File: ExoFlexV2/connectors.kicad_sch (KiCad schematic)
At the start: 12 parts, among them J10 Conn_01x03_Male, J11 Conn_01x05_Male, J12 Conn_01x03_Male, J13 Conn_01x05_Male, J14 Conn_01x03_Male, J15 Conn_01x04_Male, J16 Conn_01x09_Male, J17 Conn_01x08_Male, J18 Conn_01x04_Male, J19 Conn_01x09_Male, J8 Conn_01x03_Male, J9 Conn_01x05_Male

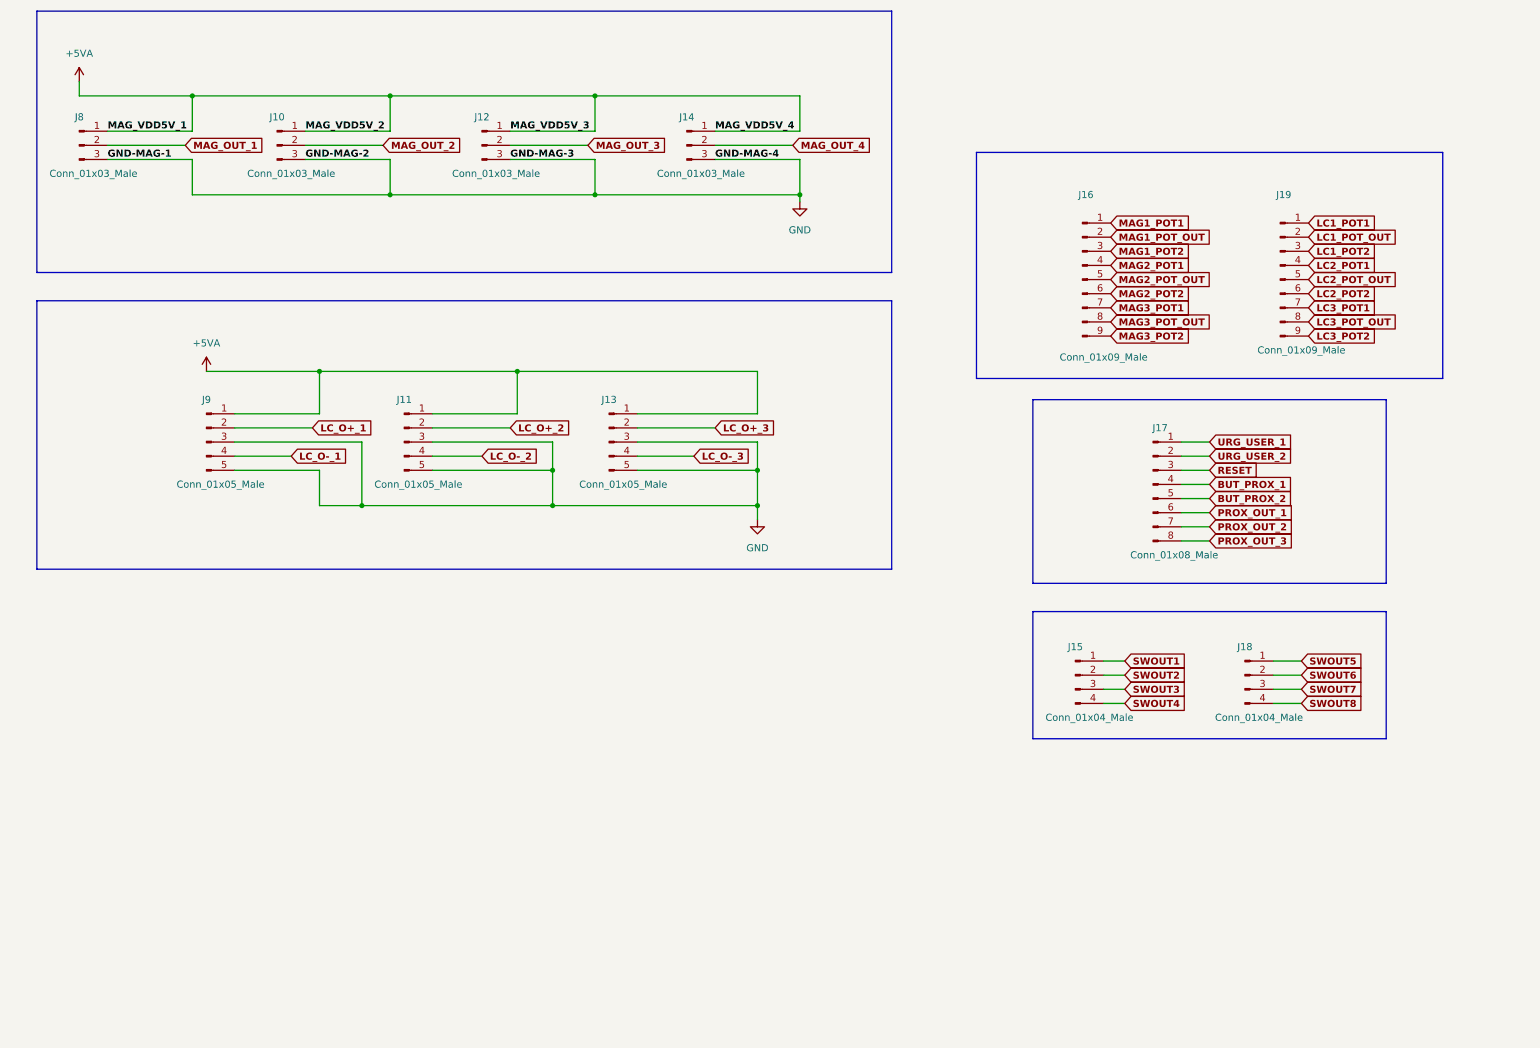
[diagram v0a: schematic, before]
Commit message: quque truc
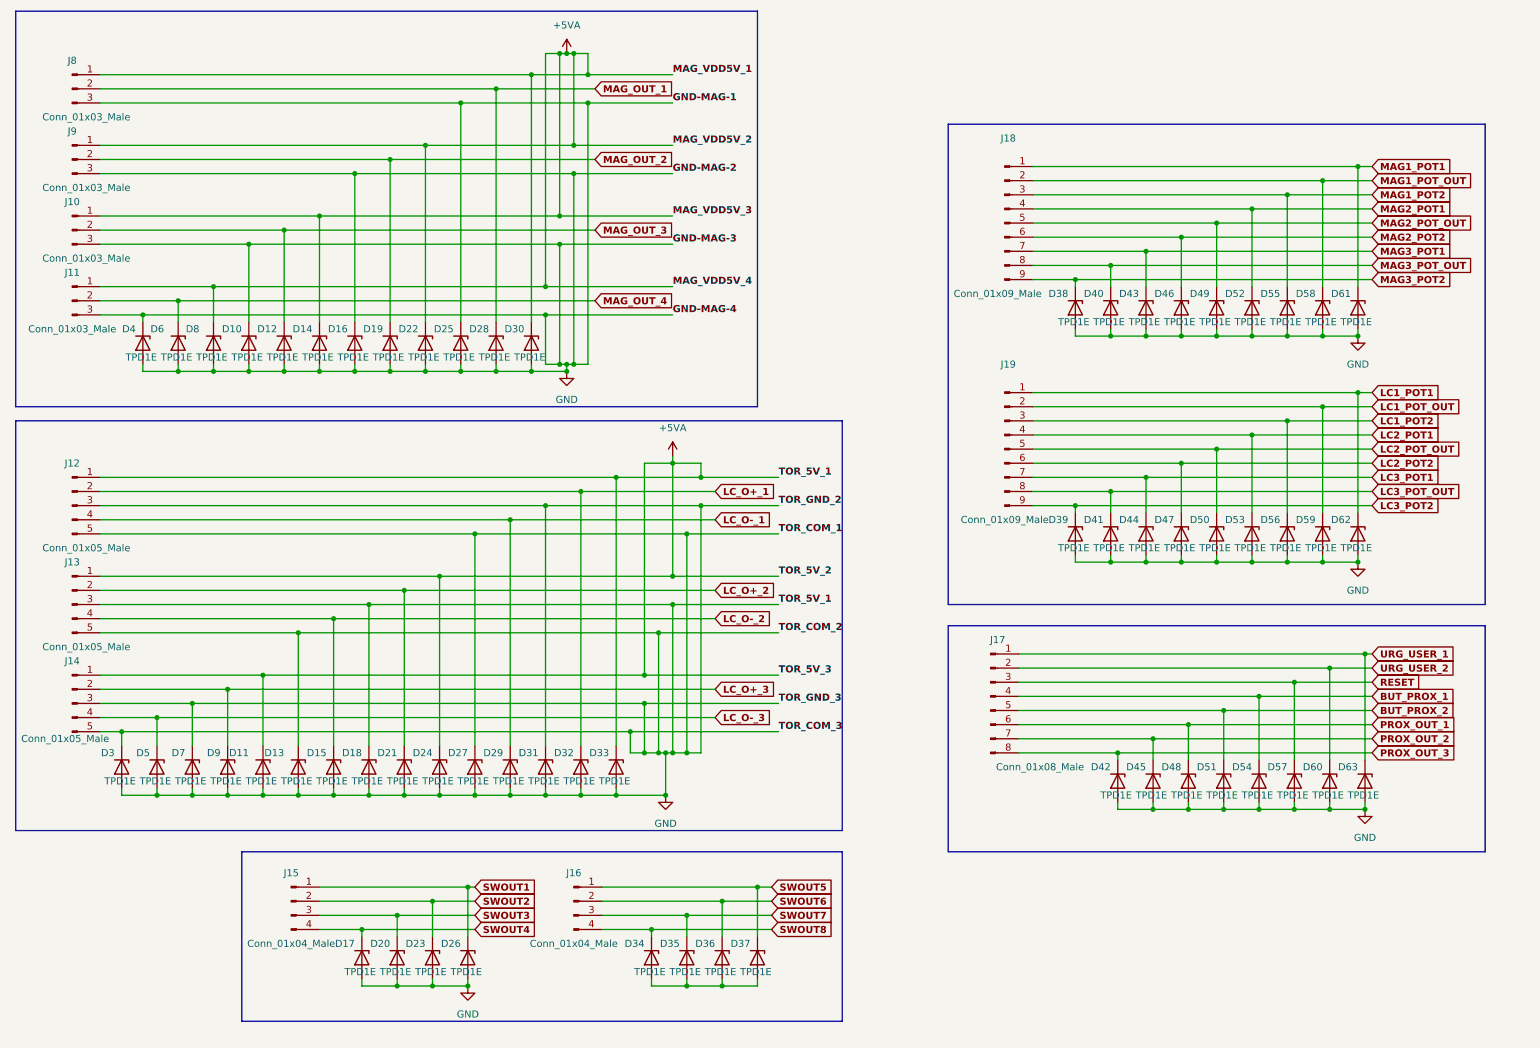
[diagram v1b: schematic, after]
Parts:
- added D10, D11, D12, D13, D14, D15, D16, D17, D18, D19, D20, D21, D22, D23, D24, D25, D26, D27, D28, D29, D3, D30, D31, D32, D33, D34, D35, D36, D37, D38, D39, D4, D40, D41, D42, D43, D44, D45, D46, D47, D48, D49, D5, D50, D51, D52, D53, D54, D55, D56, D57, D58, D59, D6, D60, D61, D62, D63, D7, D8, D9: TPD1E, FootPrint:DPY2_TEX, symbol Device:D_Zener
- J12: renamed from J9; footprint (none) -> Connector_PinHeader_2.54mm:PinHeader_1x05_P2.54mm_Vertical
- J13: renamed from J11; footprint (none) -> Connector_PinHeader_2.54mm:PinHeader_1x05_P2.54mm_Vertical
- J14: renamed from J13; footprint (none) -> Connector_PinHeader_2.54mm:PinHeader_1x05_P2.54mm_Vertical
- renumbered J12 to J10, J14 to J11, J18 to J16, J16 to J18, J10 to J9
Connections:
- net GND is gone; now on net +5VA: J10.3 (Pin_3), J11.3 (Pin_3), J12.3 (Pin_3), J12.5 (Pin_5), J13.3 (Pin_3), J13.5 (Pin_5), J14.3 (Pin_3), J14.5 (Pin_5), J8.3 (Pin_3), J9.3 (Pin_3)
- net +5VA: now also D10.1 (K), D10.2 (A), D11.1 (K), D11.2 (A), D12.2 (A), D13.1 (K), D13.2 (A), D14.1 (K), D14.2 (A), D15.2 (A), D16.1 (K), D16.2 (A), D17.2 (A), D18.1 (K), D18.2 (A), D19.2 (A), D20.2 (A), D21.2 (A), D22.1 (K), D22.2 (A), D23.2 (A), D24.1 (K), D24.2 (A), D25.1 (K), D25.2 (A), D26.2 (A), D27.1 (K), D27.2 (A), D28.2 (A), D29.2 (A), D3.1 (K), D3.2 (A), D30.1 (K), D30.2 (A), D31.1 (K), D31.2 (A), D32.2 (A), D33.1 (K), D33.2 (A), D38.2 (A), D39.2 (A), D4.1 (K), D4.2 (A), D40.2 (A), D41.2 (A), D42.2 (A), D43.2 (A), D44.2 (A), D45.2 (A), D46.2 (A), D47.2 (A), D48.2 (A), D49.2 (A), D5.2 (A), D50.2 (A), D51.2 (A), D52.2 (A), D53.2 (A), D54.2 (A), D55.2 (A), D56.2 (A), D57.2 (A), D58.2 (A), D59.2 (A), D6.2 (A), D60.2 (A), D61.2 (A), D62.2 (A), D63.2 (A), D7.1 (K), D7.2 (A), D8.1 (K), D8.2 (A), D9.2 (A)
- net BUT_PROX_1: now also D54.1 (K)
- net BUT_PROX_2: now also D51.1 (K)
- net LC1_POT1: now also D62.1 (K)
- net LC1_POT2: now also D56.1 (K)
- net LC1_POT_OUT: now also D59.1 (K)
- net LC2_POT1: now also D53.1 (K)
- net LC2_POT2: now also D47.1 (K)
- net LC2_POT_OUT: now also D50.1 (K)
- net LC3_POT1: now also D44.1 (K)
- net LC3_POT2: now also D39.1 (K)
- net LC3_POT_OUT: now also D41.1 (K)
- net LC_O+_1: now also D32.1 (K)
- net LC_O+_2: now also D21.1 (K)
- net LC_O+_3: now also D9.1 (K)
- net LC_O-_1: now also D29.1 (K)
- net LC_O-_2: now also D15.1 (K)
- net LC_O-_3: now also D5.1 (K)
- net MAG1_POT1: now also D61.1 (K)
- net MAG1_POT2: now also D55.1 (K)
- net MAG1_POT_OUT: now also D58.1 (K)
- net MAG2_POT1: now also D52.1 (K)
- net MAG2_POT2: now also D46.1 (K)
- net MAG2_POT_OUT: now also D49.1 (K)
- net MAG3_POT1: now also D43.1 (K)
- net MAG3_POT2: now also D38.1 (K)
- net MAG3_POT_OUT: now also D40.1 (K)
- net MAG_OUT_1: now also D28.1 (K)
- net MAG_OUT_2: now also D19.1 (K)
- net MAG_OUT_3: now also D12.1 (K)
- net MAG_OUT_4: now also D6.1 (K)
- net PROX_OUT_1: now also D48.1 (K)
- net PROX_OUT_2: now also D45.1 (K)
- net PROX_OUT_3: now also D42.1 (K)
- net RESET: now also D57.1 (K)
- net SWOUT1: now also D26.1 (K)
- net SWOUT2: now also D23.1 (K)
- net SWOUT3: now also D20.1 (K)
- net SWOUT4: now also D17.1 (K)
- net SWOUT5: now also D37.1 (K)
- net SWOUT6: now also D36.1 (K)
- net SWOUT7: now also D35.1 (K)
- net SWOUT8: now also D34.1 (K)
- net URG_USER_1: now also D63.1 (K)
- net URG_USER_2: now also D60.1 (K)
- new net: D34.2 (A), D35.2 (A), D36.2 (A), D37.2 (A)
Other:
- moved on the sheet: J10, J11, J12, J13, J14, J15, J16, J17, J18, J19, J8, J9

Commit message: Placement
Début du placement et modification d'après dernier review
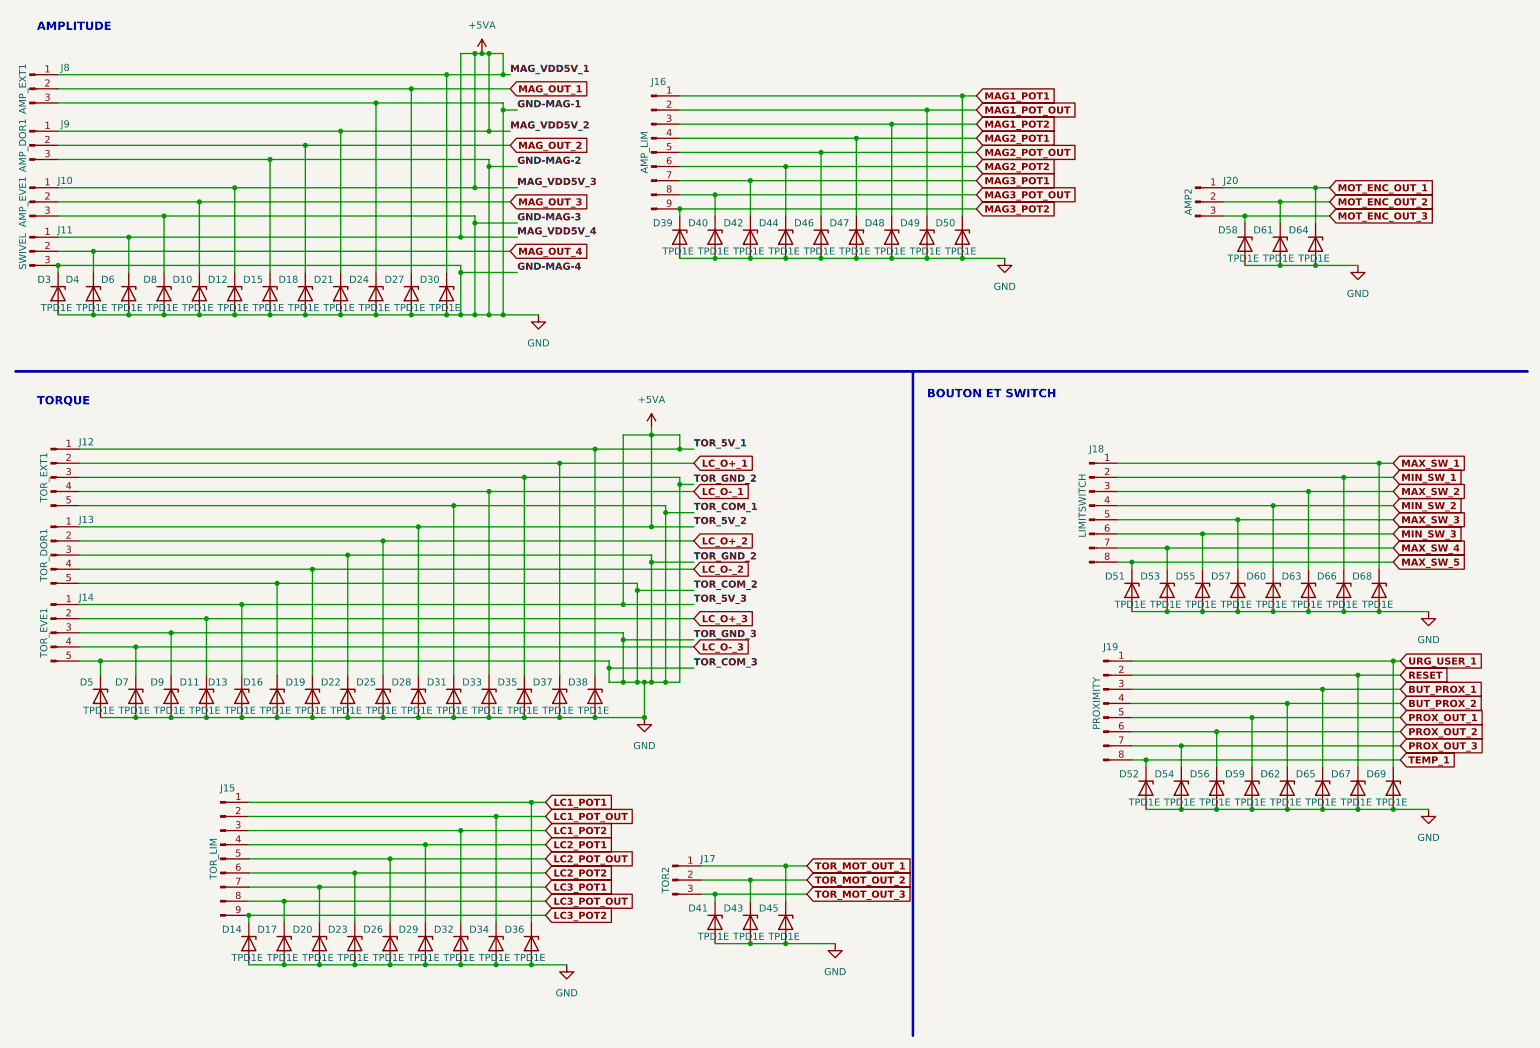
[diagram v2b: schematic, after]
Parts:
- removed D17, D20, D23, D26, D34, D35, D36, D37: TPD1E, FootPrint:DPY2_TEX, symbol Device:D_Zener
- removed J15, J16: Conn_01x04_Male, Connector_PinHeader_2.54mm:PinHeader_1x04_P2.54mm_Vertical, symbol Connector:Conn_01x04_Male
- added D41, D43, D45, D51, D53, D55, D57, D58, D60, D61, D63, D64, D66, D68: TPD1E, FootPrint:DPY2_TEX, symbol Device:D_Zener
- added J17: TOR2, Connector_PinHeader_2.54mm:PinHeader_1x03_P2.54mm_Vertical, symbol Connector:Conn_01x03_Male
- added J18: LIMITSWITCH, Connector_PinHeader_2.54mm:PinHeader_1x08_P2.54mm_Vertical, symbol Connector:Conn_01x08_Male
- added J20: AMP2, Connector_PinHeader_2.54mm:PinHeader_1x03_P2.54mm_Vertical, symbol Connector:Conn_01x03_Male
- J10: value Conn_01x03_Male -> AMP_EVE1
- J11: value Conn_01x03_Male -> SWIVEL
- J12: value Conn_01x05_Male -> TOR_EXT1
- J13: value Conn_01x05_Male -> TOR_DOR1
- J14: value Conn_01x05_Male -> TOR_EVE1
- J15: renamed from J19; value Conn_01x09_Male -> TOR_LIM
- J16: renamed from J18; value Conn_01x09_Male -> AMP_LIM
- J19: renamed from J17; value Conn_01x08_Male -> PROXIMITY
- J8: value Conn_01x03_Male -> AMP_EXT1
- J9: value Conn_01x03_Male -> AMP_DOR1
- renumbered D12 to D10, D9 to D11, D14 to D12, D11 to D13, D39 to D14, D16 to D15, D13 to D16, D41 to D17, D19 to D18, D15 to D19, D44 to D20, D22 to D21, D18 to D22, D47 to D23, D25 to D24, D21 to D25, D50 to D26, D28 to D27, D24 to D28, D53 to D29, D4 to D3, D27 to D31, D56 to D32, D29 to D33, D59 to D34, D31 to D35, D62 to D36, D32 to D37, D33 to D38, D38 to D39, D6 to D4, D43 to D42, D46 to D44, D49 to D46, D52 to D47, D55 to D48, D58 to D49, D3 to D5, D61 to D50, D42 to D52, D45 to D54, D48 to D56, D51 to D59, D8 to D6, D54 to D62, D57 to D65, D60 to D67, D63 to D69, D5 to D7, D10 to D8, D7 to D9
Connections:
- net URG_USER_2 is gone; now on net RESET: D67.1 (K), J19.2 (Pin_2)
- net +5VA: no longer D10.2 (A), D11.2 (A), D12.2 (A), D13.2 (A), D14.2 (A), D15.1 (K), D15.2 (A), D16.1 (K), D16.2 (A), D17.2 (A), D18.2 (A), D19.2 (A), D20.2 (A), D21.2 (A), D22.1 (K), D22.2 (A), D23.2 (A), D24.1 (K), D24.2 (A), D25.2 (A), D26.2 (A), D27.2 (A), D28.2 (A), D29.2 (A), D3.1 (K), D3.2 (A), D30.2 (A), D31.1 (K), D31.2 (A), D32.2 (A), D33.2 (A), D34.2 (A), D35.1 (K), D35.2 (A), D36.2 (A), D37.2 (A), D38.2 (A), D39.2 (A), D4.2 (A), D40.2 (A), D42.2 (A), D44.2 (A), D46.2 (A), D47.2 (A), D48.2 (A), D49.2 (A), D5.1 (K), D5.2 (A), D50.2 (A), D52.2 (A), D54.2 (A), D56.2 (A), D59.2 (A), D6.2 (A), D62.2 (A), D65.2 (A), D67.2 (A), D69.2 (A), D7.2 (A), D8.1 (K), D8.2 (A), D9.1 (K), D9.2 (A), J10.3 (Pin_3), J11.3 (Pin_3), J12.3 (Pin_3), J12.5 (Pin_5), J13.3 (Pin_3), J13.5 (Pin_5), J14.3 (Pin_3), J14.5 (Pin_5), J8.3 (Pin_3), J9.3 (Pin_3)
- net BUT_PROX_1: now also D65.1 (K), J19.3 (Pin_3); no longer D62.1 (K), J19.4 (Pin_4)
- net BUT_PROX_2: now also D62.1 (K), J19.4 (Pin_4); no longer D59.1 (K), J19.5 (Pin_5)
- net PROX_OUT_1: now also D59.1 (K), J19.5 (Pin_5); no longer D56.1 (K), J19.6 (Pin_6)
- net PROX_OUT_2: now also D56.1 (K), J19.6 (Pin_6); no longer D54.1 (K), J19.7 (Pin_7)
- net PROX_OUT_3: now also D54.1 (K), J19.7 (Pin_7); no longer D52.1 (K), J19.8 (Pin_8)
- net RESET: no longer D65.1 (K), J19.3 (Pin_3)
- new net GND: D10.2 (A), D11.2 (A), D12.2 (A), D13.2 (A), D14.2 (A), D15.1 (K), D15.2 (A), D16.1 (K), D16.2 (A), D17.2 (A), D18.2 (A), D19.2 (A), D20.2 (A), D21.2 (A), D22.1 (K), D22.2 (A), D23.2 (A), D24.1 (K), D24.2 (A), D25.2 (A), D26.2 (A), D27.2 (A), D28.2 (A), D29.2 (A), D3.1 (K), D3.2 (A), D30.2 (A), D31.1 (K), D31.2 (A), D32.2 (A), D33.2 (A), D34.2 (A), D35.1 (K), D35.2 (A), D36.2 (A), D37.2 (A), D38.2 (A), D39.2 (A), D4.2 (A), D40.2 (A), D41.2 (A), D42.2 (A), D43.2 (A), D44.2 (A), D45.2 (A), D46.2 (A), D47.2 (A), D48.2 (A), D49.2 (A), D5.1 (K), D5.2 (A), D50.2 (A), D51.2 (A), D52.2 (A), D53.2 (A), D54.2 (A), D55.2 (A), D56.2 (A), D57.2 (A), D58.2 (A), D59.2 (A), D6.2 (A), D60.2 (A), D61.2 (A), D62.2 (A), D63.2 (A), D64.2 (A), D65.2 (A), D66.2 (A), D67.2 (A), D68.2 (A), D69.2 (A), D7.2 (A), D8.1 (K), D8.2 (A), D9.1 (K), D9.2 (A), J10.3 (Pin_3), J11.3 (Pin_3), J12.3 (Pin_3), J12.5 (Pin_5), J13.3 (Pin_3), J13.5 (Pin_5), J14.3 (Pin_3), J14.5 (Pin_5), J8.3 (Pin_3), J9.3 (Pin_3)
- new net MAX_SW_1: D68.1 (K), J18.1 (Pin_1)
- new net MAX_SW_2: D63.1 (K), J18.3 (Pin_3)
- new net MAX_SW_3: D57.1 (K), J18.5 (Pin_5)
- new net MAX_SW_4: D53.1 (K), J18.7 (Pin_7)
- new net MAX_SW_5: D51.1 (K), J18.8 (Pin_8)
- new net MIN_SW_1: D66.1 (K), J18.2 (Pin_2)
- new net MIN_SW_2: D60.1 (K), J18.4 (Pin_4)
- new net MIN_SW_3: D55.1 (K), J18.6 (Pin_6)
- new net MOT_ENC_OUT_1: D64.1 (K), J20.1 (Pin_1)
- new net MOT_ENC_OUT_2: D61.1 (K), J20.2 (Pin_2)
- new net MOT_ENC_OUT_3: D58.1 (K), J20.3 (Pin_3)
- new net TEMP_1: D52.1 (K), J19.8 (Pin_8)
- new net TOR_MOT_OUT_1: D45.1 (K), J17.1 (Pin_1)
- new net TOR_MOT_OUT_2: D43.1 (K), J17.2 (Pin_2)
- new net TOR_MOT_OUT_3: D41.1 (K), J17.3 (Pin_3)
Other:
- note added: "AMPLITUDE"
- note added: "BOUTON ET SWITCH"
- note added: "TORQUE"
- moved on the sheet: D10, D11, D12, D13, D14, D15, D16, D17, D18, D19, D20, D21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
